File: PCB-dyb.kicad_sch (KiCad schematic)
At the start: 19 parts, among them J1 Conn_01x10, J2 Conn_01x10, SW1 SW_SPDT, U49 TPS7A20xxxDBV

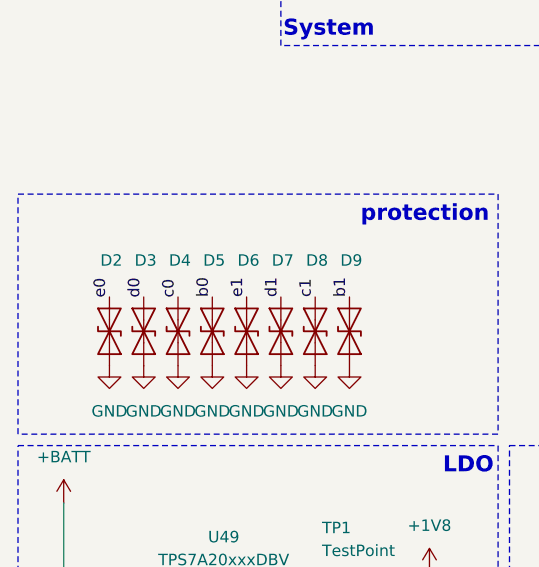
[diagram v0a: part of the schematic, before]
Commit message: add footprint
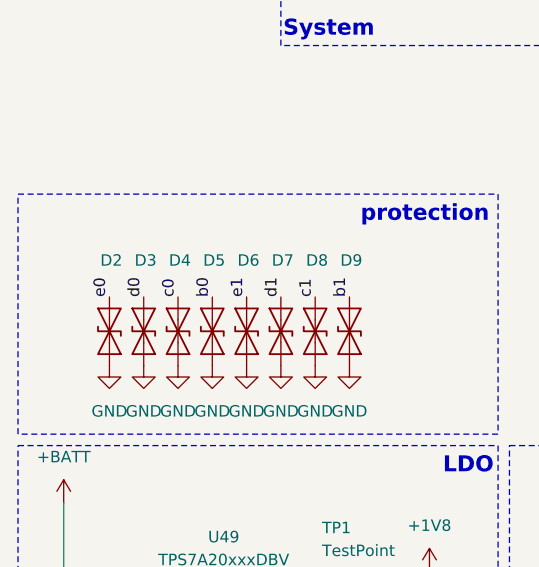
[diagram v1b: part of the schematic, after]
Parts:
- C17, C37: footprint (none) -> Capacitor_SMD:C_0603_1608Metric
- J1, J2: footprint (none) -> Connector_PinHeader_2.54mm:PinHeader_1x10_P2.54mm_Vertical; Basic (none) -> X
- SW1: footprint (none) -> Button_Switch_SMD:SW_SPDT_Shouhan_MSK12C02
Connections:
- net c0: now also D4.2 (A2)
- net d0: now also D3.2 (A2)
- net e0: now also D2.2 (A2)
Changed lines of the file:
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@@
 	)
 	(label "d0"
-		(at 26.67 146.0989 90)
+		(at 26.67 146.05 90)
 		(effects
 			(font
@@
 	)
 	(label "e0"
-		(at 22.86 146.0989 90)
+		(at 22.86 146.05 90)
 		(effects
 			(font
@@
 	)
 	(label "c0"
-		(at 30.48 146.0989 90)
+		(at 30.48 146.05 90)
 		(effects
 			(font
@@
 			)
 		)
-		(property "Footprint" ""
+		(property "Footprint" "Capacitor_SMD:C_0603_1608Metric"
 			(at 46.6852 187.96 0)
 			(hide yes)
@@
 			)
 		)
-		(property "Footprint" ""
+		(property "Footprint" "Capacitor_SMD:C_0603_1608Metric"
 			(at 18.7452 189.23 0)
 			(hide yes)
@@
 			)
 		)
-		(property "Footprint" ""
+		(property "Footprint" "Button_Switch_SMD:SW_SPDT_Shouhan_MSK12C02"
 			(at 101.6 175.26 0)
 			(hide yes)
@@
 			)
 		)
-		(property "Footprint" ""
+		(property "Footprint" "Connector_PinHeader_2.54mm:PinHeader_1x10_P2.54mm_Vertical"
 			(at 62.23 80.01 0)
 			(hide yes)
@@
 			)
 		)
-		(property "Basic" ""
+		(property "Basic" "X"
 			(at 62.23 80.01 0)
 			(hide yes)
@@
 			)
 		)
-		(property "Footprint" ""
+		(property "Footprint" "Connector_PinHeader_2.54mm:PinHeader_1x10_P2.54mm_Vertical"
 			(at 182.88 81.28 0)
 			(hide yes)
@@
 			)
 		)
-		(property "Basic" ""
+		(property "Basic" "X"
 			(at 182.88 81.28 0)
 			(hide yes)
